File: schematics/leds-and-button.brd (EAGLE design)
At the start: 54.3 x 27.9 mm, 14 parts, among them IC1 74LS595N

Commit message: Updated the schematics
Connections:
- net IC_VCC: now also IC1.10
- net PB2: now also IC1.11; no longer IC1.12
- net PB3: now also IC1.12; no longer IC1.11
- net PB4: no longer IC1.10
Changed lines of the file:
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@@
 <contactref element="JP3" pad="1"/>
 <contactref element="BTN" pad="2"/>
-<wire x1="25.4" y1="1.27" x2="20.32" y2="5.08" width="0" layer="19" extent="1-1"/>
+<contactref element="IC1" pad="10"/>
+<wire x1="25.4" y1="1.27" x2="41.91" y2="5.08" width="0" layer="19" extent="1-1"/>
+<wire x1="20.32" y1="5.08" x2="25.4" y2="1.27" width="0" layer="19" extent="1-1"/>
 </signal>
 <signal name="GND">
@@
 </signal>
 <signal name="PB3">
-<contactref element="IC1" pad="11"/>
 <contactref element="JP3" pad="6"/>
-<wire x1="7.62" y1="5.08" x2="41.91" y2="7.62" width="0" layer="19" extent="1-1"/>
+<contactref element="IC1" pad="12"/>
+<wire x1="7.62" y1="5.08" x2="41.91" y2="10.16" width="0" layer="19" extent="1-1"/>
 </signal>
 <signal name="PB4">
-<contactref element="IC1" pad="10"/>
 <contactref element="JP3" pad="7"/>
-<wire x1="5.08" y1="5.08" x2="41.91" y2="5.08" width="0" layer="19" extent="1-1"/>
 </signal>
 <signal name="PB2">
-<contactref element="IC1" pad="12"/>
 <contactref element="JP3" pad="5"/>
-<wire x1="10.16" y1="5.08" x2="41.91" y2="10.16" width="0" layer="19" extent="1-1"/>
+<contactref element="IC1" pad="11"/>
+<wire x1="10.16" y1="5.08" x2="41.91" y2="7.62" width="0" layer="19" extent="1-1"/>
 </signal>
 </signals>

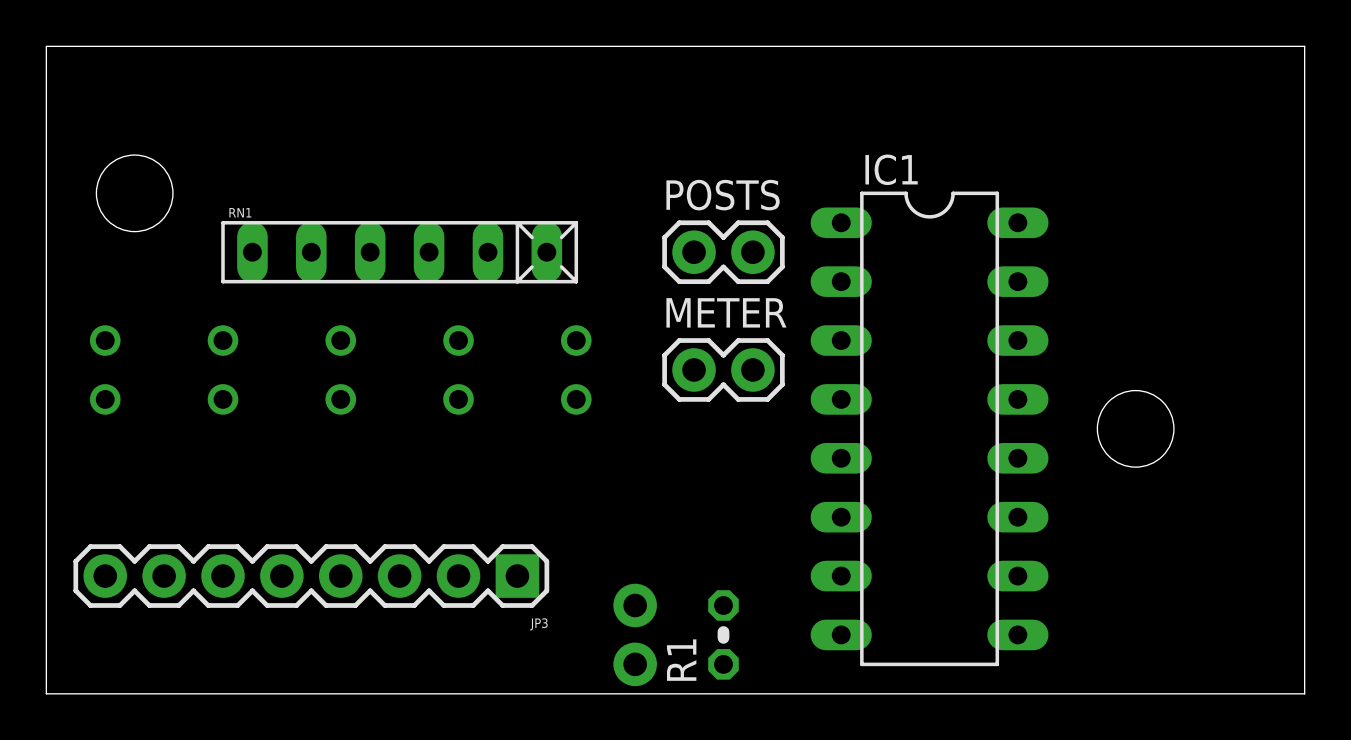
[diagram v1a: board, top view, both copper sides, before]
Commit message: Played around with the board for the leds
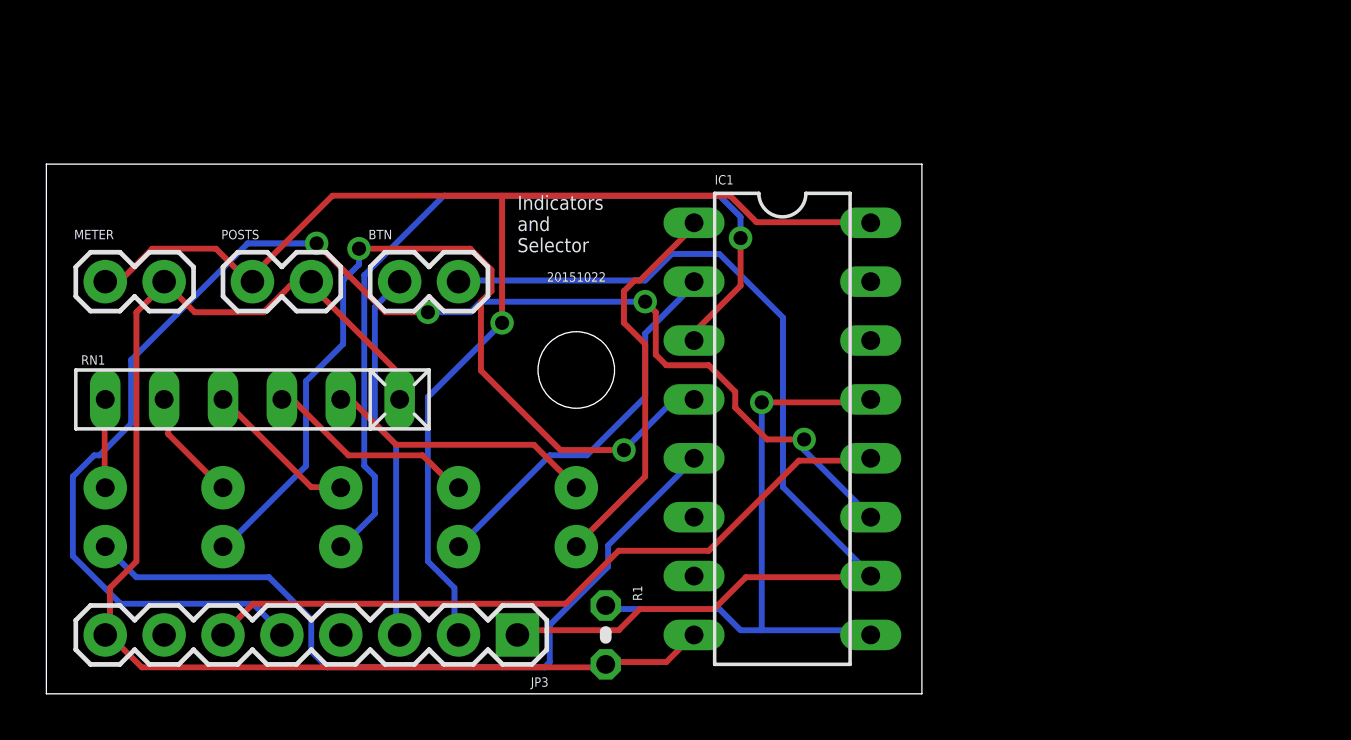
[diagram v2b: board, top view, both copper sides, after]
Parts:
- removed JP1: STAND-OFF, SparkFun:STAND-OFF
- 12V, 3.3V, 5V, 9V, ADJV: device SparkFun:LED3MM-NS -> SparkFun-LED:LED3MM
- moved METER 25.7 mm to (2.54, 17.8)
- moved JP2 20.5 mm to (22.9, 14.0)
- moved POSTS 19.1 mm to (8.89, 17.8)
- moved BTN 17.3 mm to (15.2, 17.8), flipped to the top, turned to 0 degrees
- moved RN1 8.98 mm to (8.89, 12.7)
- moved IC1 6.35 mm to (31.8, 11.4)
- moved 12V 6.35 mm to (7.62, 7.62)
- moved 3.3V 6.35 mm to (22.9, 7.62)
- moved 5V 6.35 mm to (17.8, 7.62)
- moved 9V 6.35 mm to (12.7, 7.62)
- moved ADJV 6.35 mm to (2.54, 7.62)
- moved R1 5.08 mm to (24.1, 2.54), turned to 270 degrees
- moved JP3 2.54 mm to (20.3, 2.54)
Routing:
- net PB2: track 0.00 -> 61.1 mm, vias 0 -> 4
- net VCC: track 0.00 -> 57.2 mm, vias 0 -> 1
- net GND: track 0.00 -> 56.9 mm
- net IC_VCC: track 0.00 -> 44.7 mm
- net N$5: track 0.00 -> 37.5 mm, vias 0 -> 2
- net N$6: track 0.00 -> 36.8 mm, vias 0 -> 1
- net N$4: track 0.00 -> 33.6 mm
- net PB3: track 0.00 -> 31.1 mm
- net N$11: track 0.00 -> 26.6 mm, vias 0 -> 1
- net N$13: track 0.00 -> 17.0 mm
- net N$7: track 0.00 -> 16.6 mm
- net PB0: track 0.00 -> 16.1 mm
- net N$9: track 0.00 -> 11.8 mm
- net N$8: track 0.00 -> 9.19 mm
- net N$3: track 0.00 -> 6.64 mm
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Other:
- board size 54.3 x 27.9 mm -> 37.8 x 22.9 mm
- board text added: "20151022"
- board text added: "Indicators and Selector"
